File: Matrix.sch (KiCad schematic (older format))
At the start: 3 parts

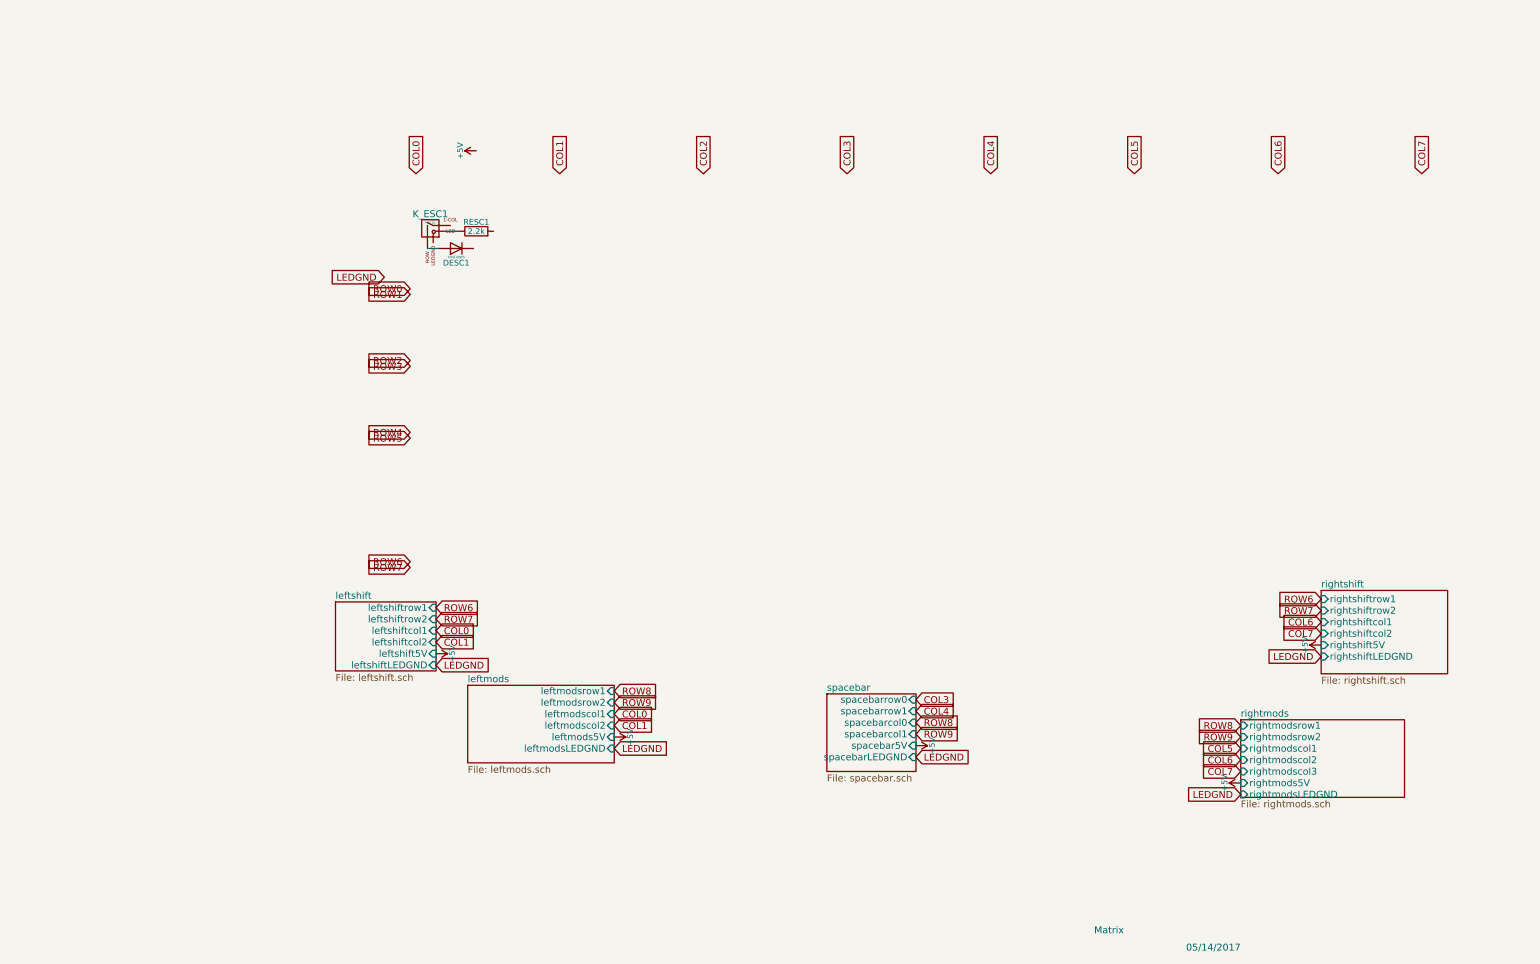
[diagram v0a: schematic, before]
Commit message: Clone a bunch of keys
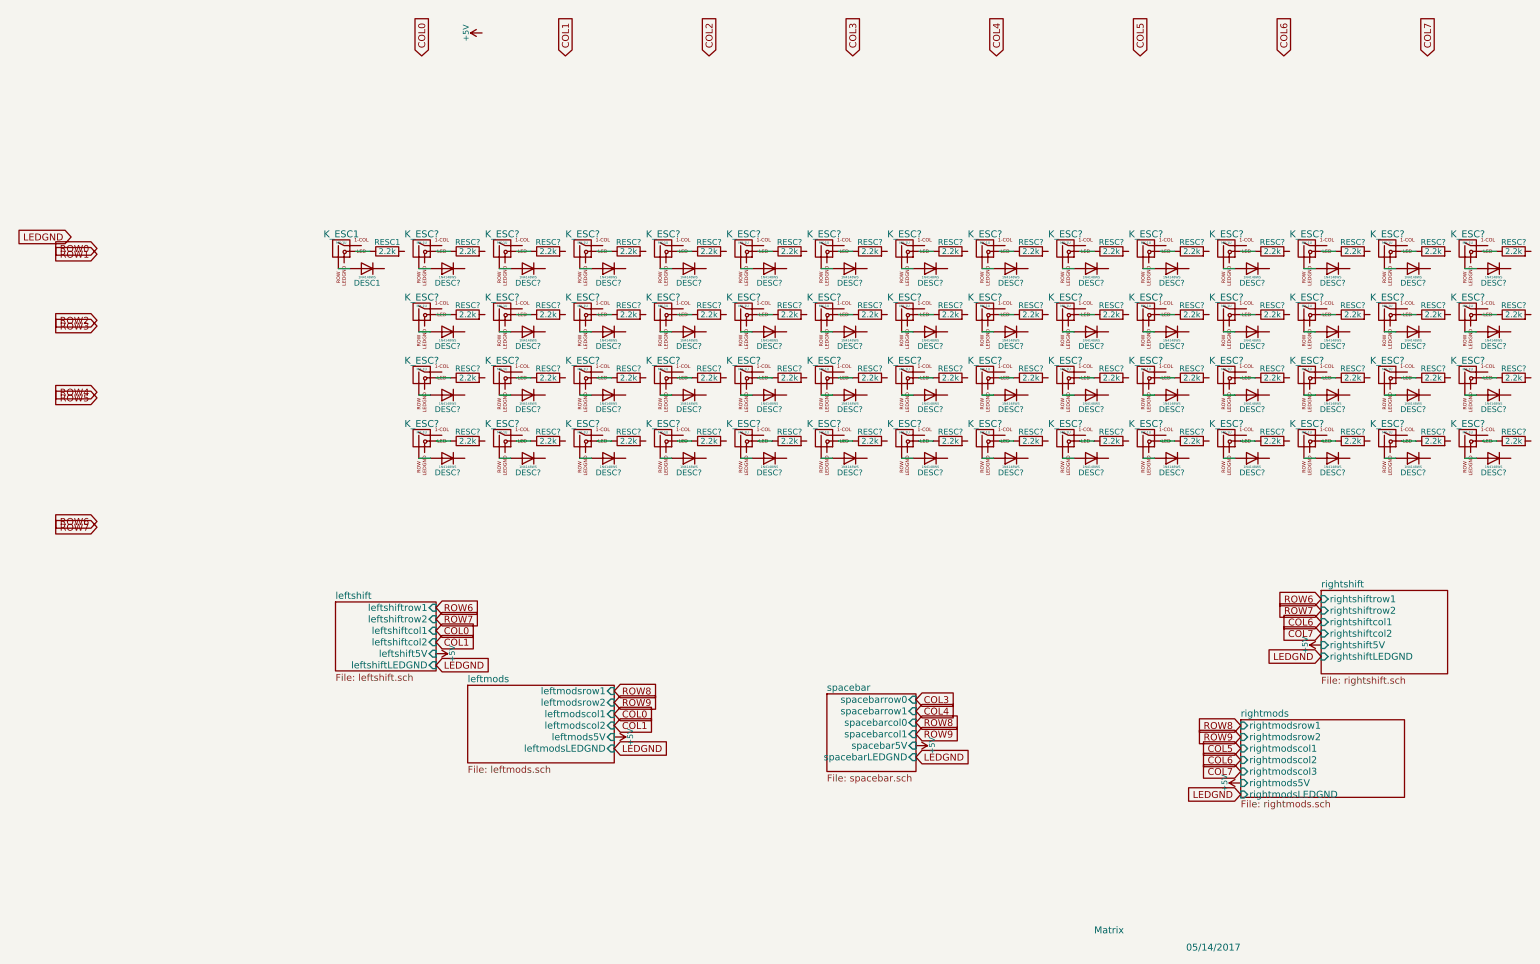
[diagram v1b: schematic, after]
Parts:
- added DESC? (x56): 1N4148WS, symbol D
- added K_ESC? (x56): MX-1U, MX_Alps_Hybrid:MX-1U, symbol MX-1U
- added RESC? (x56): 2.2k, symbol R
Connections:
- new net: DESC?.2 (A), K_ESC?.2 (ROW) (x56)
- new net: K_ESC?.3 (LED), RESC?.1 (x56)
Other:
- moved on the sheet: DESC1, K_ESC1, RESC1
